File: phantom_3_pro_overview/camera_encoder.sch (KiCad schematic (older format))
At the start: 7 parts

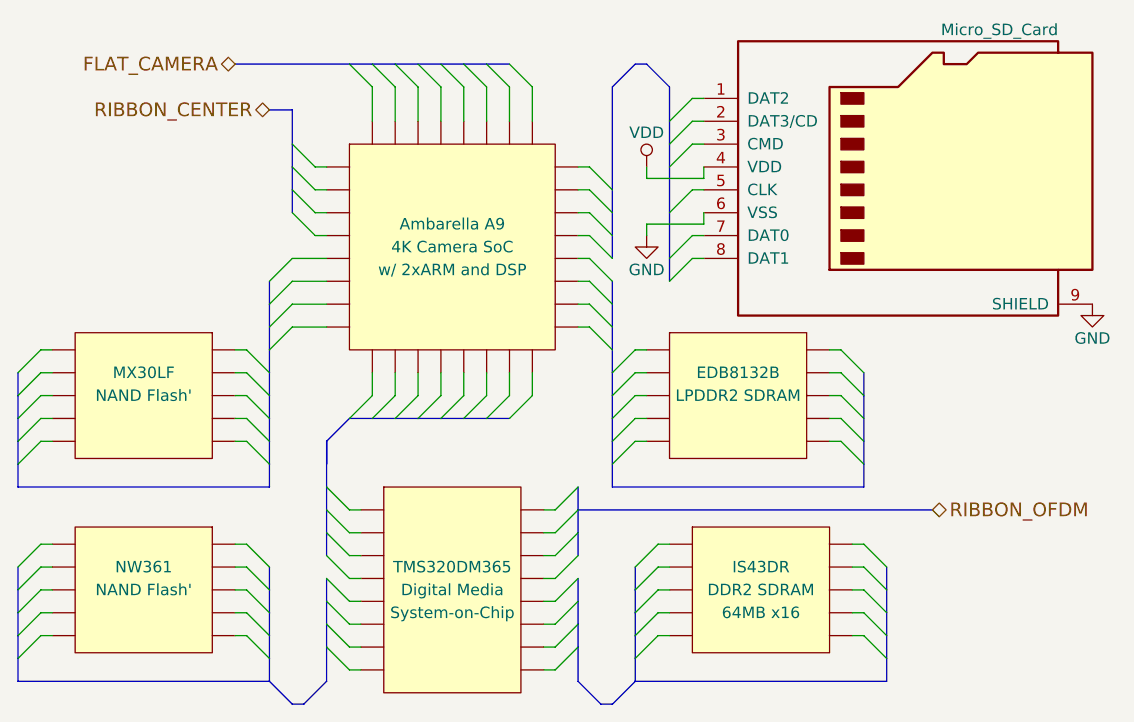
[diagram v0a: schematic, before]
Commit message: Overview: Started work on camera sensor brd.
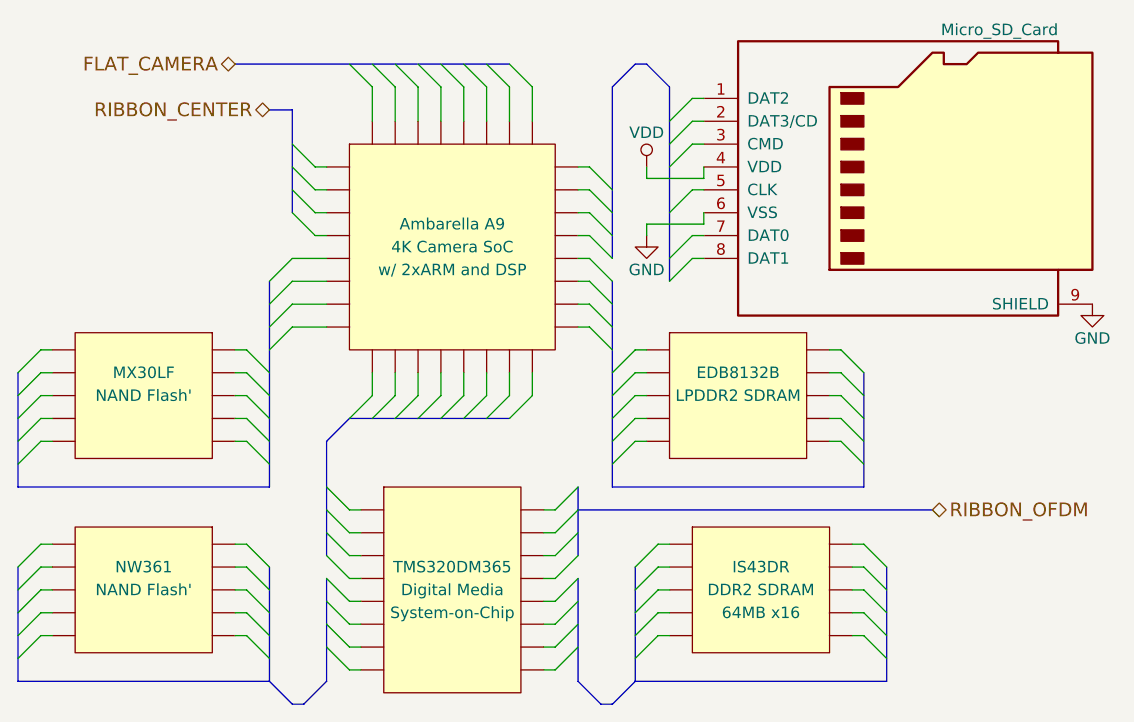
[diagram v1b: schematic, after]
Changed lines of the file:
@@
 LIBS:transistors-switches
 LIBS:transistors-power
+LIBS:sensors-v2
+LIBS:regul-v2
 LIBS:phantom_3_pro_overview-cache
 EELAYER 25 0
@@
 	1750 1850 1900 1850
 Wire Bus Line
-	3400 800  3400 950
-Wire Bus Line
-	3400 950  3400 1050
-Wire Bus Line
-	3400 1050 3400 1150
-Wire Bus Line
-	3400 1150 3400 1350
-Wire Bus Line
-	3400 1350 3400 1550
-Wire Bus Line
-	3400 1550 3400 1650
-Wire Bus Line
-	1500 700  2000 700
-Wire Bus Line
-	2000 700  2100 700
-Wire Bus Line
-	2100 700  2200 700
-Wire Bus Line
-	2200 700  2300 700
-Wire Bus Line
-	2300 700  2400 700
-Wire Bus Line
-	2400 700  2500 700
-Wire Bus Line
-	2500 700  2600 700
-Wire Bus Line
-	2600 700  2700 700
+	3400 800  3400 1650
+Wire Bus Line
+	1500 700  2700 700
 Wire Bus Line
 	3250 700  3300 700
@@
 	2000 2650 1900 2550
 Wire Bus Line
-	1900 2350 1900 2450
-Wire Bus Line
-	1900 2350 1900 2550
-Wire Bus Line
-	1900 2550 1900 2650
-Wire Bus Line
-	1900 2650 1900 2750
-Wire Bus Line
-	1900 2750 1900 2850
+	1900 2350 1900 2850
 Entry Wire Line
 	2900 3350 3000 3250
@@
 	2900 2650 3000 2550
 Wire Bus Line
-	1750 900  1750 1050
-Wire Bus Line
-	1750 1050 1750 1150
-Wire Bus Line
-	1750 1150 1750 1250
-Wire Bus Line
-	1750 1250 1750 1350
+	1750 900  1750 1350
 Wire Wire Line
 	2000 2650 2050 2650
@@
 	3150 3500 3250 3400
 Wire Bus Line
-	3250 2900 3250 3000
-Wire Bus Line
-	3250 3000 3250 3100
-Wire Bus Line
-	3250 3100 3250 3200
-Wire Bus Line
-	3250 3200 3250 3300
-Wire Bus Line
-	3250 3300 3250 3400
+	3250 2900 3250 3400
 Wire Bus Line
 	3100 3500 3150 3500
@@
 	3400 3200 3350 3200
 Wire Bus Line
-	4350 2900 4350 3000
-Wire Bus Line
-	4350 3000 4350 3100
-Wire Bus Line
-	4350 3100 4350 3200
-Wire Bus Line
-	4350 3200 4350 3300
-Wire Bus Line
-	4350 3300 4350 3400
+	4350 2900 4350 3400
 Wire Bus Line
 	4350 3400 3250 3400
 Wire Bus Line
-	3000 2550 3000 2650
-Wire Bus Line
-	3000 2650 3000 2750
-Wire Bus Line
-	3000 2750 3000 2850
-Wire Bus Line
-	3000 2950 3000 3050
-Wire Bus Line
-	3000 3050 3000 3150
-Wire Bus Line
-	3000 3150 3000 3250
-Wire Bus Line
-	3000 3250 3000 3400
+	3000 2550 3000 2850
+Wire Bus Line
+	3000 2950 3000 3400
 $Comp
 L IC_DIL10 U?
@@
 	1750 3500 1650 3400
 Wire Bus Line
-	1650 2900 1650 3000
-Wire Bus Line
-	1650 3000 1650 3100
-Wire Bus Line
-	1650 3100 1650 3200
-Wire Bus Line
-	1650 3200 1650 3300
-Wire Bus Line
-	1650 3300 1650 3400
+	1650 2900 1650 3400
 Wire Bus Line
 	1800 3500 1750 3500
@@
 	1500 3200 1550 3200
 Wire Bus Line
-	550  2900 550  3000
-Wire Bus Line
-	550  3000 550  3100
-Wire Bus Line
-	550  3100 550  3200
-Wire Bus Line
-	550  3200 550  3300
-Wire Bus Line
-	550  3300 550  3400
+	550  2900 550  3400
 Wire Bus Line
 	550  3400 1650 3400
 Wire Bus Line
-	1900 2950 1900 3050
-Wire Bus Line
-	1900 3050 1900 3150
-Wire Bus Line
-	1900 3150 1900 3250
-Wire Bus Line
-	1900 3250 1900 3400
+	1900 2950 1900 3400
 $Comp
 L IC_DIL10 U?
@@
 $EndComp
 Wire Bus Line
-	3150 1650 3150 1750
-Wire Bus Line
-	3150 1750 3150 1850
-Wire Bus Line
-	3150 1850 3150 1950
-Wire Bus Line
-	3150 1950 3150 2050
-Wire Bus Line
-	3150 2050 3150 2150
-Wire Bus Line
-	3150 2150 3150 2250
-Wire Bus Line
-	3150 2250 3150 2350
-Wire Bus Line
-	3150 2350 3150 2450
-Wire Bus Line
-	3150 2450 3150 2550
+	3150 1650 3150 2550
 Entry Wire Line
 	4250 2450 4150 2350
@@
 	3300 2350 3250 2350
 Wire Bus Line
-	4250 2050 4250 2150
-Wire Bus Line
-	4250 2150 4250 2250
-Wire Bus Line
-	4250 2250 4250 2350
-Wire Bus Line
-	4250 2350 4250 2450
-Wire Bus Line
-	4250 2450 4250 2550
+	4250 2050 4250 2550
 Wire Bus Line
 	4250 2550 3150 2550
 Wire Bus Line
-	3150 800  3150 800
-Wire Bus Line
-	3150 800  3150 1250
-Wire Bus Line
-	3150 1250 3150 1350
-Wire Bus Line
-	3150 1350 3150 1450
-Wire Bus Line
-	3150 1450 3150 1550
+	3150 800  3150 1550
 Wire Bus Line
 	3000 2650 4550 2650
@@
 $EndComp
 Wire Bus Line
-	1650 1650 1650 1750
-Wire Bus Line
-	1650 1750 1650 1850
-Wire Bus Line
-	1650 1850 1650 1950
-Wire Bus Line
-	1650 1950 1650 2050
-Wire Bus Line
-	1650 2050 1650 2150
-Wire Bus Line
-	1650 2150 1650 2250
-Wire Bus Line
-	1650 2250 1650 2350
-Wire Bus Line
-	1650 2350 1650 2450
-Wire Bus Line
-	1650 2450 1650 2550
+	1650 1650 1650 2550
 Entry Wire Line
 	550  2450 650  2350
@@
 	1500 2350 1550 2350
 Wire Bus Line
-	550  2050 550  2150
-Wire Bus Line
-	550  2150 550  2250
-Wire Bus Line
-	550  2250 550  2350
-Wire Bus Line
-	550  2350 550  2450
-Wire Bus Line
-	550  2450 550  2550
+	550  2050 550  2550
 Wire Bus Line
 	550  2550 1650 2550
 Wire Bus Line
-	2000 2250 2100 2250
-Wire Bus Line
-	2100 2250 2200 2250
-Wire Bus Line
-	2200 2250 2300 2250
-Wire Bus Line
-	2300 2250 2400 2250
-Wire Bus Line
-	2400 2250 2500 2250
-Wire Bus Line
-	2500 2250 2600 2250
-Wire Bus Line
-	2600 2250 2700 2250
+	2000 2250 2700 2250
 Entry Bus Bus
 	1900 2350 2000 2250
